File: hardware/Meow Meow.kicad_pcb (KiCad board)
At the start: 2 copper layers, 93 x 57.5 mm, 45 parts, among them J3 SWD, P1 SPACE, P10 A, P11 W, P12 KEY_UP_ARROW, P2 KEY_DOWN_ARROW, P3 KEY_RIGHT_ARROW, P5 KEY_LEFT_ARROW, P6 D, P7 S, P8 MOUSE_LEFT, SW1 RESET, U1 ATSAMD11D14A-SS, U2 AP2112K-3.3

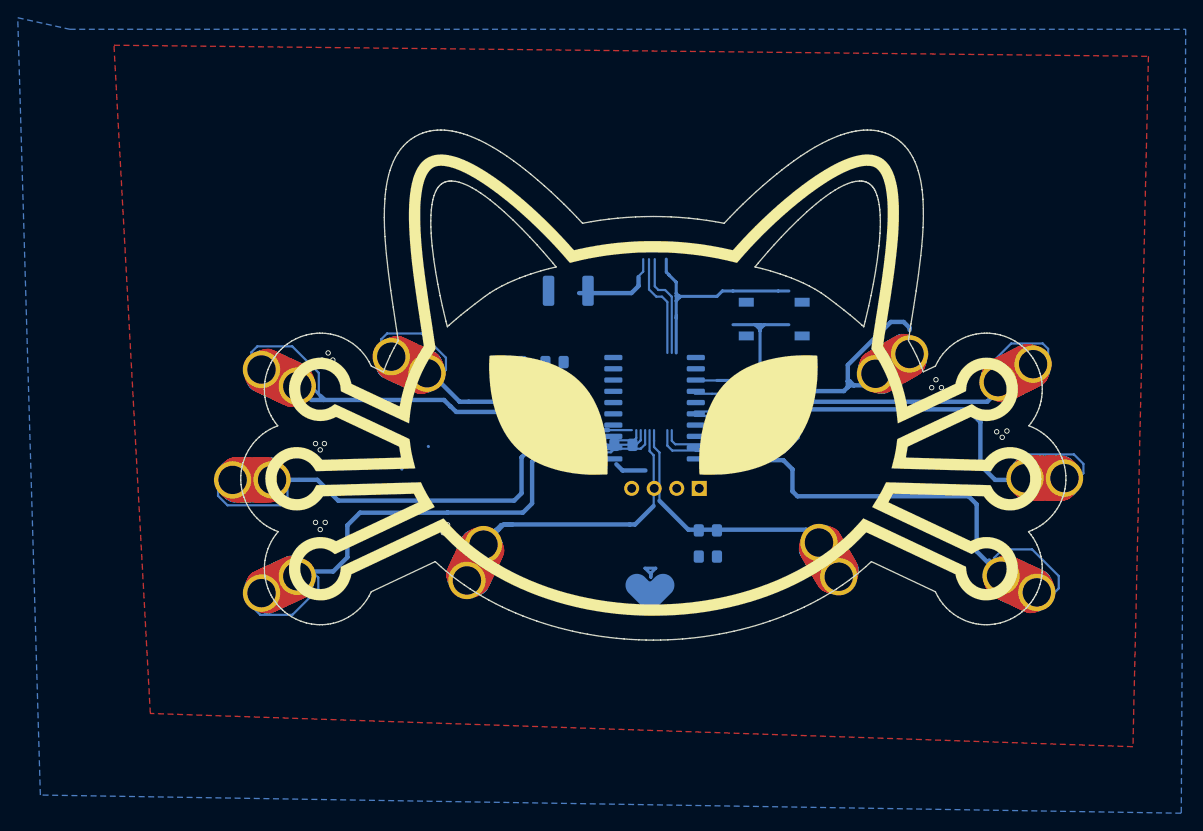
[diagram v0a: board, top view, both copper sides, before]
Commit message: Update size
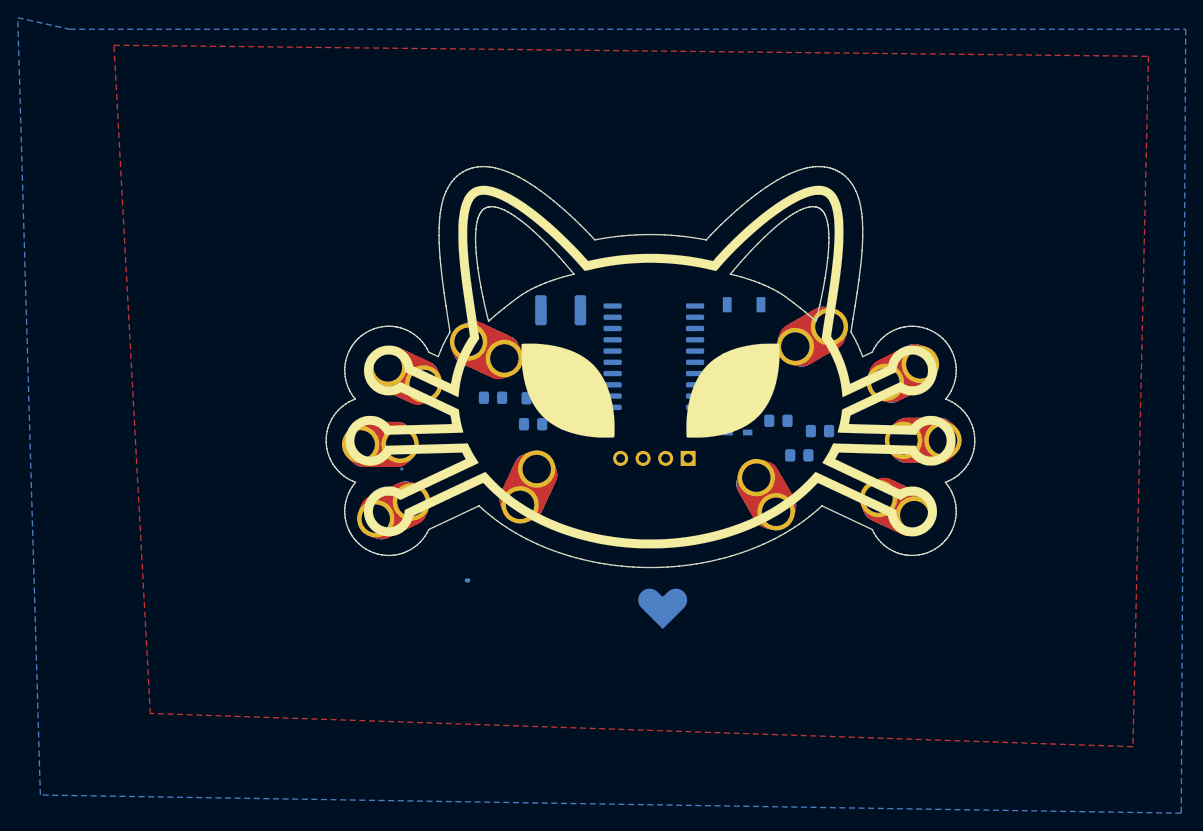
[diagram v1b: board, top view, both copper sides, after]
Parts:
- removed the G*** at (142.9, 101.6)
- removed the G*** at (142.7, 129.0)
- moved G*** 48.4 mm to (124.1, 137.2)
- moved C2 19.0 mm to (161.7, 115.6)
- moved G*** 18.6 mm to (115.6, 136.9)
- moved P6 16.3 mm to (170.4, 124.2)
- moved P5 15.4 mm to (113.4, 124.5)
- moved P3 15.0 mm to (112.2, 117.1)
- moved P7 14.3 mm to (173.4, 116.6)
- moved P2 14.3 mm to (115.1, 109.4)
- moved C5 13.3 mm to (159.3, 118.3)
- moved P10 12.7 mm to (171.2, 109.0)
- moved D2 11.6 mm to (124.8, 111.8)
- moved P1 10.4 mm to (128.9, 121.7)
- moved P8 10.2 mm to (155.6, 122.9)
- moved P11 9.54 mm to (160.7, 105.0)
- moved P12 8.88 mm to (124.2, 106.5)
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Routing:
- net /Y2: track 67.3 -> 0.00 mm
- net /Y3: track 66.9 -> 0.00 mm
- net /Y0: track 66.2 -> 0.00 mm
- net /Y1: track 64.1 -> 4.81 mm
- net /Y4: track 57.4 -> 0.00 mm
- net /Y9: track 54.5 -> 0.00 mm
- net /Y5: track 40.2 -> 0.00 mm
- net /Y8: track 37.0 -> 0.00 mm
- net /Y15: track 34.5 -> 0.15 mm
- net GND: track 29.3 -> 0.00 mm, vias 18 -> 0
- net /Y14: track 28.1 -> 0.00 mm
- net /SWDIO: track 21.9 -> 0.00 mm
- net /D-: track 16.6 -> 0.00 mm
- net /D+: track 11.8 -> 0.00 mm
- net Net-(F1-Pad2): track 10.5 -> 0.00 mm
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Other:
- board size 93 x 57.5 mm -> 73.1 x 45.2 mm
- board text removed: "X3"
- board text removed: "X7"
